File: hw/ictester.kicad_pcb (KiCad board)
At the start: 4 copper layers, 78.2 x 91.4 mm, 71 parts, among them J1 Conn_01x12_Pin, J2 Conn_01x12_Pin, J3 Conn_01x01_Pin, J4 Conn_01x01_Pin, J6 Conn_01x06_Pin, J7 Conn_01x04_Pin, J8 Conn_02x05_Odd_Even, J9 USB_B_Micro, U1 ATmega1284-A, U2 CP2102N-Axx-xQFN28, U3 CDSOT236-0504C, U4 MAX14662, U5 MAX14662, U6 MAX14662, U7 MAX14662, U8 MAX14662, U9 ZIF24, Y1 20MHz

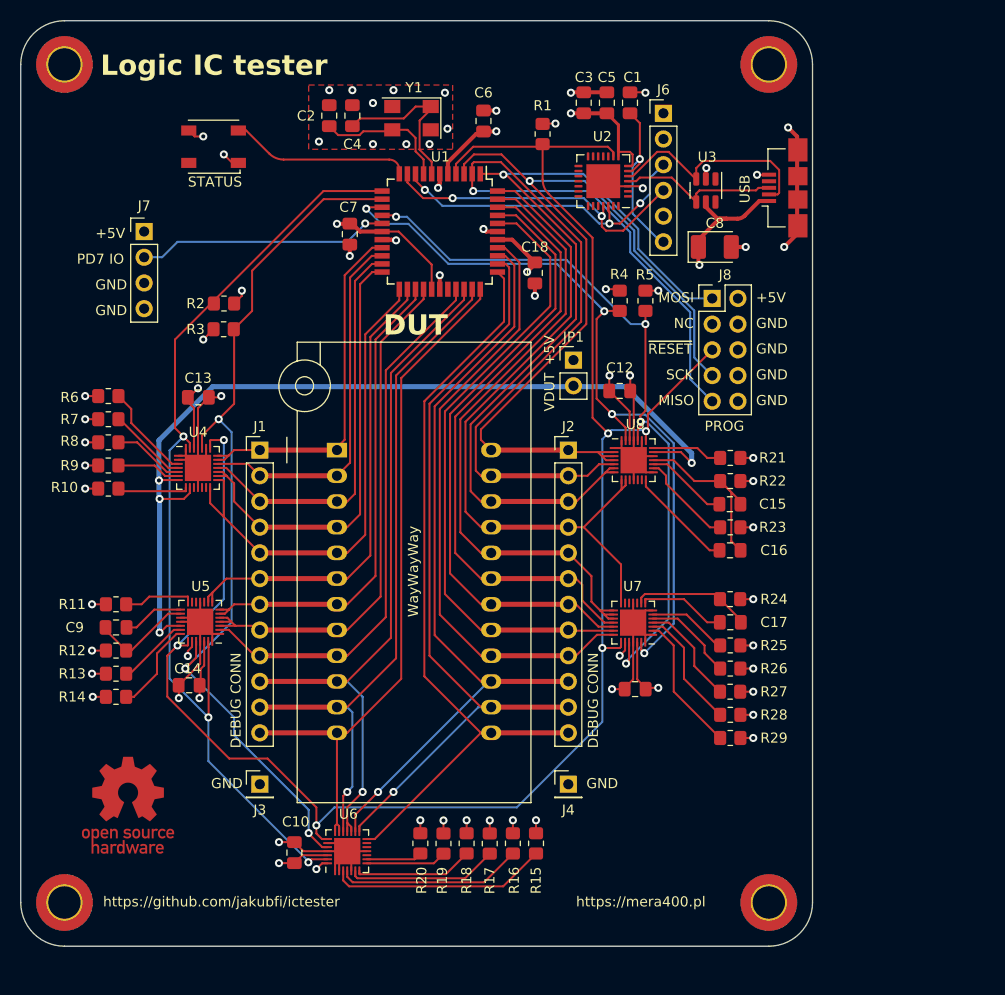
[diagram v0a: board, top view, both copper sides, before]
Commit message: H/W v3
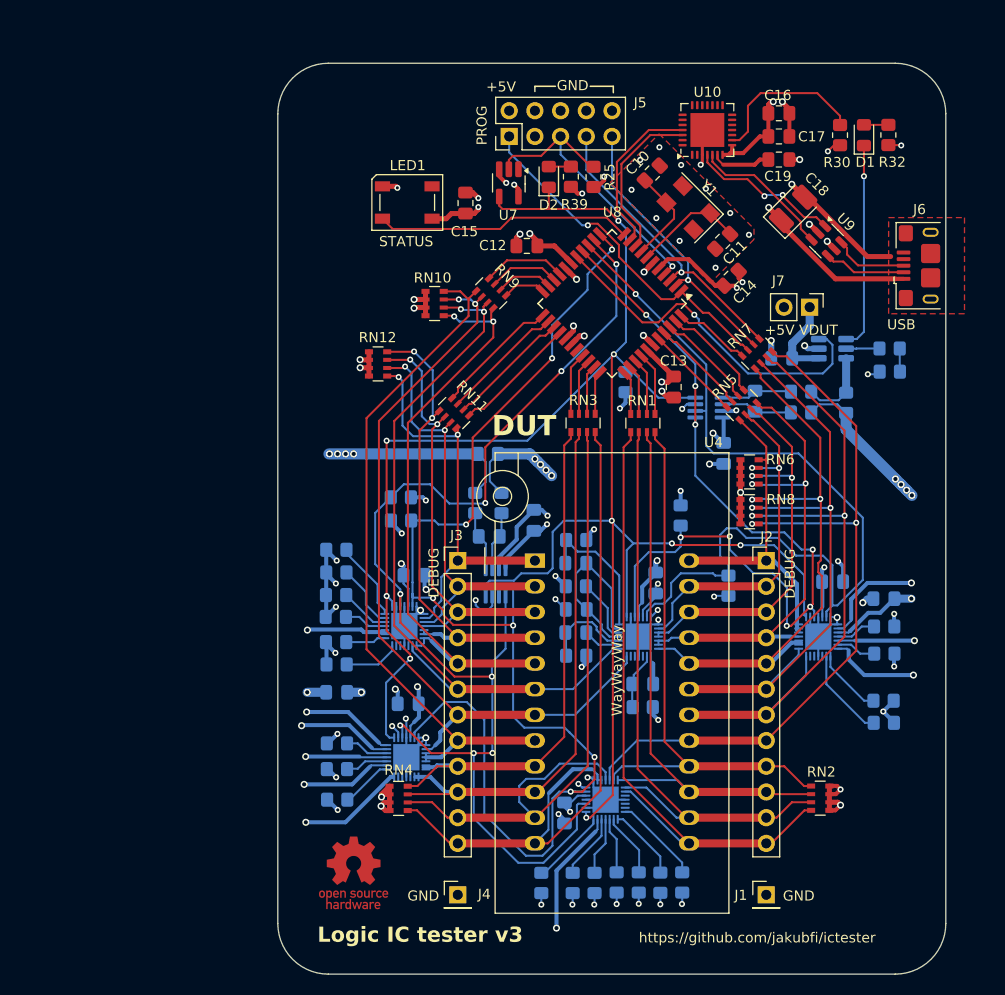
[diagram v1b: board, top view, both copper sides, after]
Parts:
- removed H1, H2, H3, H4: MountingHole_Pad, MountingHole:MountingHole_3.2mm_M3_DIN965_Pad_TopBottom
- removed J8: Conn_02x05_Odd_Even, Connector_PinHeader_2.54mm:PinHeader_2x05_P2.54mm_Vertical
- removed J9: USB_B_Micro, Connector_USB:USB_Micro-B_Amphenol_10104110_Horizontal
- removed JP1: Jumper_2_Open, Connector_PinHeader_2.54mm:PinHeader_1x02_P2.54mm_Vertical
- added C19: 100n, Capacitor_SMD:C_0805_2012Metric_Pad1.18x1.45mm_HandSolder, F.Cu at (176.5, 64.5)
- added C20: 100n, Capacitor_SMD:C_0805_2012Metric_Pad1.18x1.45mm_HandSolder, B.Cu at (176.8, 84.2)
- added C21: 1u, Capacitor_SMD:C_0805_2012Metric_Pad1.18x1.45mm_HandSolder, B.Cu at (186.9, 107.9)
- added C22: 1u, Capacitor_SMD:C_0805_2012Metric_Pad1.18x1.45mm_HandSolder, B.Cu at (132.8, 117.2)
- added C23: 100n, Capacitor_SMD:C_0805_2012Metric_Pad1.18x1.45mm_HandSolder, B.Cu at (174.2, 88.4)
- added C24: 100n, Capacitor_SMD:C_0805_2012Metric_Pad1.18x1.45mm_HandSolder, B.Cu at (147.9, 101.8)
- added C25: 100n, Capacitor_SMD:C_0805_2012Metric_Pad1.18x1.45mm_HandSolder, B.Cu at (171.1, 93.5)
- added C26: 100n, Capacitor_SMD:C_0805_2012Metric_Pad1.18x1.45mm_HandSolder, B.Cu at (152.3, 100.2)
- added D1: RED, LED_SMD:LED_0805_2012Metric_Pad1.15x1.40mm_HandSolder, F.Cu at (184.9, 62.1)
- added D2: ORANGE, LED_SMD:LED_0805_2012Metric_Pad1.15x1.40mm_HandSolder, F.Cu at (153.8, 66.2)
- added J5: Conn_02x05_Odd_Even, Connector_PinHeader_2.54mm:PinHeader_2x05_P2.54mm_Vertical, F.Cu at (149.9, 62.2)
- added R30: 4k7, Resistor_SMD:R_0805_2012Metric_Pad1.20x1.40mm_HandSolder, F.Cu at (182.6, 62.1)
- added R31: 133k, Resistor_SMD:R_0805_2012Metric_Pad1.20x1.40mm_HandSolder, B.Cu at (187.5, 83.2)
- added R32: 1k0, Resistor_SMD:R_0805_2012Metric_Pad1.20x1.40mm_HandSolder, F.Cu at (187.3, 62.1)
- added R33: 200m, Resistor_SMD:R_0805_2012Metric_Pad1.20x1.40mm_HandSolder, B.Cu at (183.2, 88.5)
- added R34: 200m, Resistor_SMD:R_0805_2012Metric_Pad1.20x1.40mm_HandSolder, B.Cu at (147.8, 93.6)
- added R35: 47, Resistor_SMD:R_0805_2012Metric_Pad1.20x1.40mm_HandSolder, B.Cu at (178.7, 87.5)
- added R36: 47, Resistor_SMD:R_0805_2012Metric_Pad1.20x1.40mm_HandSolder, B.Cu at (178.7, 89.5)
- added R37: 47, Resistor_SMD:R_0805_2012Metric_Pad1.20x1.40mm_HandSolder, B.Cu at (146.5, 98.5)
- added R38: 47, Resistor_SMD:R_0805_2012Metric_Pad1.20x1.40mm_HandSolder, B.Cu at (149.1, 98.5)
- added R39: 1k0, Resistor_SMD:R_0805_2012Metric_Pad1.20x1.40mm_HandSolder, F.Cu at (156.0, 66.2)
- added R40: 4k7, Resistor_SMD:R_0805_2012Metric_Pad1.20x1.40mm_HandSolder, B.Cu at (161.3, 86.5)
- added R41: 0, Resistor_SMD:R_0805_2012Metric_Pad1.20x1.40mm_HandSolder, B.Cu at (187.5, 85.5)
- added RN1: 120, Resistor_SMD:R_Array_Convex_4x0603, F.Cu at (163.1, 90.6)
- added RN10: 1M, Resistor_SMD:R_Array_Convex_4x0603, F.Cu at (142.5, 78.7)
- added RN11: 120, Resistor_SMD:R_Array_Convex_4x0603, F.Cu at (144.4, 89.6)
- added RN12: 1M, Resistor_SMD:R_Array_Convex_4x0603, F.Cu at (136.9, 84.7)
- added RN2: 1M, Resistor_SMD:R_Array_Convex_4x0603, F.Cu at (180.6, 127.6)
- added RN3: 120, Resistor_SMD:R_Array_Convex_4x0603, F.Cu at (157.2, 90.5)
- added RN4: 1M, Resistor_SMD:R_Array_Convex_4x0603, F.Cu at (138.9, 127.6)
- added RN5: 120, Resistor_SMD:R_Array_Convex_4x0603, F.Cu at (172.8, 88.8)
- added RN6: 1M, Resistor_SMD:R_Array_Convex_4x0603, F.Cu at (173.6, 95.4)
- added RN7: 120, Resistor_SMD:R_Array_Convex_4x0603, F.Cu at (174.4, 83.7)
- added RN8: 1M, Resistor_SMD:R_Array_Convex_4x0603, F.Cu at (173.6, 99.3)
- added RN9: 120, Resistor_SMD:R_Array_Convex_4x0603, F.Cu at (148.1, 77.7)
- added U10: CP2102N, Package_DFN_QFN:QFN-28-1EP_5x5mm_P0.5mm_EP3.35x3.35mm, F.Cu at (169.4, 61.6)
- added U11: TPS2553, Package_TO_SOT_SMD:SOT-23-6_Handsoldering, B.Cu at (181.8, 83.2)
- added U12: INA236, Package_TO_SOT_SMD:SOT-23-8_Handsoldering, B.Cu at (169.6, 89.0)
- added U13: INA236, Package_TO_SOT_SMD:SOT-23-8_Handsoldering, B.Cu at (148.5, 106.2)
- C1, R10, R11, R12, R13, R14, R15, R16, R17, R18, R19, R2, R20, R21, R22, R23, R24, R26, R27, R28, R29, R3, R4, R5, R6, R7, R8, R9, U5, U6: moved to B.Cu
- C10, C11: value 100n -> 22p
- C15, C17: value 470p -> 100n
- C16: value 470p -> 1u
- C18: value 100n -> 10u; footprint Capacitor_SMD:C_0805_2012Metric_Pad1.18x1.45mm_HandSolder -> Capacitor_Tantalum_SMD:CP_EIA-3528-21_Kemet-B_Pad1.50x2.35mm_HandSolder
- C2, C4: value 22p -> 100n; moved to B.Cu
- C3, C6, C7: value 100n -> 470p; moved to B.Cu
- C5: value 1u -> 100p; moved to B.Cu
- C8: value 10u -> 100n; footprint Capacitor_Tantalum_SMD:CP_EIA-3528-21_Kemet-B_Pad1.50x2.35mm_HandSolder -> Capacitor_SMD:C_0805_2012Metric_Pad1.18x1.45mm_HandSolder; moved to B.Cu
- C9: value 470p -> 100n; moved to B.Cu
- J1: value Conn_01x12_Pin -> Conn_01x01_Pin; footprint Connector_PinHeader_2.54mm:PinHeader_1x12_P2.54mm_Vertical -> Connector_PinHeader_2.54mm:PinHeader_1x01_P2.54mm_Vertical
- J3: value Conn_01x01_Pin -> Conn_01x12_Pin; footprint Connector_PinHeader_2.54mm:PinHeader_1x01_P2.54mm_Vertical -> Connector_PinHeader_2.54mm:PinHeader_1x12_P2.54mm_Vertical
- J6: value Conn_01x06_Pin -> USB_B_Micro; footprint Connector_PinHeader_2.54mm:PinHeader_1x06_P2.54mm_Vertical -> Connector_USB:USB_Micro-B_Amphenol_10118193-0001LF_Horizontal
- J7: value Conn_01x04_Pin -> Conn_02x01; footprint Connector_PinHeader_2.54mm:PinHeader_1x04_P2.54mm_Vertical -> Connector_PinHeader_2.54mm:PinHeader_1x02_P2.54mm_Vertical
- R1: value 10k -> 4k7; moved to B.Cu
- R25: value 4k7 -> 10k
- U1: value ATmega1284-A -> MAX14662; footprint Package_QFP:TQFP-44_10x10mm_P0.8mm -> Package_DFN_QFN:QFN-28-1EP_4x4mm_P0.4mm_EP2.6x2.6mm; moved to B.Cu
- U2: value CP2102N-Axx-xQFN28 -> MAX14662; footprint Package_DFN_QFN:QFN-28-1EP_5x5mm_P0.5mm_EP3.35x3.35mm -> Package_DFN_QFN:QFN-28-1EP_4x4mm_P0.4mm_EP2.6x2.6mm; moved to B.Cu
- U3: value CDSOT236-0504C -> MAX14662; footprint Package_TO_SOT_SMD:SOT-23-6 -> Package_DFN_QFN:QFN-28-1EP_4x4mm_P0.4mm_EP2.6x2.6mm; moved to B.Cu
- U4: value MAX14662 -> ZIF24; footprint Package_DFN_QFN:QFN-28-1EP_4x4mm_P0.4mm_EP2.6x2.6mm -> Socket:DIP_Socket-24_W11.9_W12.7_W15.24_W17.78_W18.5_3M_224-1275-00-0602J
- U7: value MAX14662 -> 74LVC1G07; footprint Package_DFN_QFN:QFN-28-1EP_4x4mm_P0.4mm_EP2.6x2.6mm -> Package_TO_SOT_SMD:SOT-23-5_HandSoldering
- U8: value MAX14662 -> ATmega1284-A; footprint Package_DFN_QFN:QFN-28-1EP_4x4mm_P0.4mm_EP2.6x2.6mm -> Package_QFP:TQFP-44_10x10mm_P0.8mm
- U9: value ZIF24 -> USBLC6-2SC6; footprint Socket:DIP_Socket-24_W11.9_W12.7_W15.24_W17.78_W18.5_3M_224-1275-00-0602J -> Package_TO_SOT_SMD:SOT-23-6
- moved C10 75.9 mm to (164.0, 65.8), turned to 45 degrees
- moved R3 74.8 mm to (186.9, 118.0)
- moved R2 73.9 mm to (186.9, 113.3), turned to 0 degrees
- moved C2 72.7 mm to (155.3, 129.1)
- moved C14 67.0 mm to (171.8, 76.2), turned to -135 degrees
- moved J1 66.6 mm to (175.3, 137.2)
- moved J7 66.2 mm to (179.6, 79.1), turned to -90 degrees
- moved R10 65.3 mm to (162.7, 135.9), turned to -90 degrees
- moved R9 65.0 mm to (160.5, 135.9), turned to -90 degrees
- moved R7 64.8 mm to (156.1, 136.0), turned to -90 degrees
- moved R8 64.8 mm to (158.3, 136.0), turned to -90 degrees
- moved R6 64.4 mm to (153.0, 136.0), turned to -90 degrees
- moved U2 61.1 mm to (159.4, 127.8), turned to -90 degrees
- moved R12 60.5 mm to (167.0, 135.9), turned to -90 degrees
- moved R11 60.4 mm to (164.8, 136.0), turned to -90 degrees
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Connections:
- C1 pad 1: Net-(J6-Pin_6) -> +5V
- C10 pad 1: +5V -> Net-(U8-XTAL1)
- C11 pad 1: +5V -> GND
- C11 pad 2: GND -> Net-(U8-XTAL2)
- C12 pad 1: +5V -> GND
- C12 pad 2: GND -> +5V
- C13 pad 1: +5V -> GND
- C13 pad 2: GND -> +5V
- C14 pad 1: +5V -> GND
- C14 pad 2: GND -> +5V
- C15 pad 1: Net-(U8-B5) -> +5V
- C15 pad 2: Net-(U8-B4) -> GND
- C16 pad 1: Net-(U8-B8) -> +5V
- C16 pad 2: Net-(U8-B4) -> GND
- C17 pad 1: Net-(U7-A7) -> +5V
- C17 pad 2: Net-(U7-A8) -> GND
- C18 pad 1: GND -> +5V
- C18 pad 2: +5V -> GND
- C2 pad 1: GND -> +5V
- C2 pad 2: Net-(U1-XTAL1) -> GND
- C3 pad 1: +5V -> Net-(U3-A7)
- C3 pad 2: GND -> Net-(U3-A8)
- C4 pad 1: GND -> +5V
- C4 pad 2: Net-(U1-XTAL2) -> GND
- C5 pad 1: +5V -> GND
- C5 pad 2: GND -> Net-(U3-B2)
- C6 pad 1: GND -> Net-(U3-B1)
- C6 pad 2: +5V -> Net-(U3-B2)
- C7 pad 1: GND -> Net-(U3-B5)
- C7 pad 2: +5V -> Net-(U3-B6)
- C9 pad 1: Net-(U5-B6) -> +5V
- C9 pad 2: Net-(U5-B7) -> GND
- J1 pad 1: ZIF1 -> GND
- J3 pad 1: GND -> ZIF1
- J6 pad 2: GND -> Net-(J6-D-)
- J6 pad 3: TXD -> Net-(J6-D+)
- J6 pad 4: RXD -> unconnected-(J6-ID-Pad4)
- J6 pad 5: unconnected-(J6-Pin_5-Pad5) -> GND
- J6 pad 6: Net-(J6-Pin_6) -> GND
- J7 pad 1: +5V -> Net-(J7-Pin_1)
- J7 pad 2: Net-(J7-Pin_2) -> +5V
- R1 pad 1: +5V -> Net-(U1-A3)
- R1 pad 2: ~{RESET} -> +5V
- R10 pad 1: Net-(U4-A7) -> Net-(U2-B6)
- R11 pad 1: Net-(U5-B8) -> Net-(U2-B7)
- R12 pad 1: Net-(U5-B6) -> Net-(U2-B8)
- R13 pad 1: Net-(U5-B2) -> +5V
- R13 pad 2: +5V -> Net-(U3-B1)
- R14 pad 1: Net-(U5-B1) -> +5V
- R14 pad 2: +5V -> Net-(U3-B3)
- R15 pad 1: Net-(U6-A2) -> +5V
- R15 pad 2: +5V -> Net-(U3-B5)
- R16 pad 1: Net-(U6-A3) -> Net-(U5-B3)
- R17 pad 1: Net-(U6-A5) -> Net-(U5-B5)
- R18 pad 1: Net-(U6-A6) -> Net-(U5-B7)
- R19 pad 1: Net-(U6-A7) -> Net-(U6-B1)
- R2 pad 1: +5V -> Net-(U1-A5)
- R2 pad 2: SDA1 -> +5V
- R20 pad 1: Net-(U6-A8) -> Net-(U6-B2)
- R21 pad 1: Net-(U8-B1) -> Net-(U6-B3)
- R22 pad 1: Net-(U8-B4) -> Net-(U6-B4)
- R23 pad 1: Net-(U8-B6) -> Net-(U6-B7)
- R24 pad 1: Net-(U7-A8) -> Net-(U6-B8)
- R25 pad 1: Net-(U7-A5) -> +5V
- R25 pad 2: +5V -> Net-(J5-Pin_5)
- R26 pad 1: Net-(U7-A4) -> +5V
- R26 pad 2: +5V -> SDA1
- R27 pad 1: Net-(U7-A3) -> +5V
- R27 pad 2: +5V -> SCL1
- R28 pad 1: Net-(U7-A2) -> +5V
- R28 pad 2: +5V -> SDA2
- R29 pad 1: Net-(U7-A1) -> +5V
- R29 pad 2: +5V -> SCL2
- R3 pad 1: +5V -> Net-(U1-A7)
- R3 pad 2: SCL1 -> +5V
- R4 pad 1: +5V -> Net-(U1-A8)
- R4 pad 2: SDA2 -> +5V
- R5 pad 1: +5V -> Net-(U3-A8)
- R5 pad 2: SCL2 -> +5V
- R6 pad 1: Net-(U4-A2) -> Net-(U2-B1)
- R7 pad 1: Net-(U4-A3) -> Net-(U2-B3)
- R8 pad 1: Net-(U4-A4) -> Net-(U2-B4)
- R9 pad 1: Net-(U4-A5) -> Net-(U2-B5)
- U1 pad 1: ZIF22 -> GND
- U1 pad 10: RXD -> unconnected-(U1-NC-Pad10)
- U1 pad 11: Net-(LED1-DIN) -> GND
- U1 pad 12: SDA1 -> unconnected-(U1-NC-Pad12)
- U1 pad 13: SCL1 -> unconnected-(U1-NC-Pad13)
- U1 pad 14: SDA2 -> ZIF18
- U1 pad 15: SCL2 -> ZIF19
- U1 pad 16: Net-(J7-Pin_2) -> ZIF20
- U1 pad 17: +5V -> ZIF20
- U1 pad 18: GND -> ZIF21
- U1 pad 19: ZIF1 -> ZIF24
- U1 pad 2: ZIF23 -> GNDUT
- U1 pad 20: ZIF2 -> ZIF24
- U1 pad 21: ZIF3 -> ZIF24
- U1 pad 22: ZIF4 -> ~{SD}
- U1 pad 23: ZIF5 -> GND
- U1 pad 24: ZIF6 -> SCL2
- U1 pad 25: ZIF7 -> GND
- U1 pad 26: ZIF8 -> +5V
- U1 pad 27: +5V -> SDA2
- U1 pad 29: unconnected-(U1-AREF-Pad29) -> GND
- U1 pad 3: ZIF24 -> VDUT
- U1 pad 4: ~{RESET} -> Net-(U1-A3)
- U1 pad 5: +5V -> GNDUT
- U1 pad 6: GND -> Net-(U1-A5)
- U1 pad 7: Net-(U1-XTAL2) -> GNDUT
- U1 pad 8: Net-(U1-XTAL1) -> Net-(U1-A7)
- U1 pad 9: TXD -> Net-(U1-A8)
- U2 pad 1: unconnected-(U2-~{DCD}-Pad1) -> GND
- U2 pad 11: unconnected-(U2-~{SUSPEND}-Pad11) -> GND
- U2 pad 14: unconnected-(U2-CHR1-Pad14) -> Net-(U2-B8)
- U2 pad 15: unconnected-(U2-CHR0-Pad15) -> Net-(U2-B7)
- U2 pad 16: unconnected-(U2-~{WAKEUP}/GPIO.3-Pad16) -> Net-(U2-B6)
- U2 pad 17: unconnected-(U2-RS485/GPIO.2-Pad17) -> Net-(U2-B5)
- U2 pad 18: unconnected-(U2-~{RXT}/GPIO.1-Pad18) -> Net-(U2-B4)
- U2 pad 19: unconnected-(U2-~{TXT}/GPIO.0-Pad19) -> Net-(U2-B3)
- U2 pad 2: unconnected-(U2-~{RI}/CLK-Pad2) -> ZIF12
- U2 pad 20: unconnected-(U2-GPIO.6-Pad20) -> GNDUT
- U2 pad 21: unconnected-(U2-GPIO.5-Pad21) -> Net-(U2-B1)
- U2 pad 22: unconnected-(U2-GPIO.4-Pad22) -> ~{SD}
- U2 pad 23: unconnected-(U2-~{CTS}-Pad23) -> GND
- U2 pad 24: unconnected-(U2-~{RTS}-Pad24) -> SCL1
- U2 pad 25: RXD -> GND
- U2 pad 26: TXD -> +5V
- U2 pad 27: unconnected-(U2-~{DSR}-Pad27) -> SDA1
- U2 pad 28: unconnected-(U2-~{DTR}-Pad28) -> +5V
- U2 pad 3: GND -> ZIF12
- U2 pad 4: Net-(J9-D+) -> ZIF11
- U2 pad 5: Net-(J9-D-) -> ZIF17
- U2 pad 6: Net-(J6-Pin_6) -> ZIF16
- U2 pad 7: +5V -> ZIF15
- U2 pad 8: +5V -> ZIF14
- U2 pad 9: ~{RESET} -> ZIF13
- U3 pad 1: unconnected-(U3-IO1-Pad1) -> GND
- U3 pad 2: GND -> ZIF23
- U3 pad 3: Net-(J9-D-) -> ZIF22
- U3 pad 4: Net-(J9-D+) -> ZIF22
- U3 pad 5: +5V -> ZIF21
- U3 pad 6: unconnected-(U3-IO4-Pad6) -> ZIF21
- U4 pad 1: GND -> ZIF1
- U4 pad 10: unconnected-(U4-NC-Pad10) -> ZIF10
- U4 pad 11: GND -> ZIF11
- U4 pad 12: unconnected-(U4-NC-Pad12) -> ZIF12
- U4 pad 13: unconnected-(U4-NC-Pad13) -> ZIF13
- U4 pad 14: ZIF5 -> ZIF14
- U4 pad 15: ZIF5 -> ZIF15
- U4 pad 16: ZIF4 -> ZIF16
- U4 pad 17: ZIF4 -> ZIF17
- U4 pad 18: ZIF3 -> ZIF18
- U4 pad 19: ZIF2 -> ZIF19
- U4 pad 2: GND -> ZIF2
- U4 pad 20: ZIF1 -> ZIF20
- U4 pad 21: ZIF1 -> ZIF21
- U4 pad 22: ~{RESET} -> ZIF22
- U4 pad 23: GND -> ZIF23
- U4 pad 24: SCL1 -> ZIF24
- U4 pad 3: Net-(U4-A2) -> ZIF3
- U4 pad 4: Net-(U4-A3) -> ZIF4
- U4 pad 5: Net-(U4-A4) -> ZIF5
- U4 pad 6: Net-(U4-A5) -> ZIF6
- U4 pad 7: +5VD -> ZIF7
- U4 pad 8: Net-(U4-A7) -> ZIF8
- U4 pad 9: +5VD -> ZIF9
- U5 pad 14: Net-(U5-B8) -> GNDUT
- U5 pad 16: Net-(U5-B6) -> VDUT
- U5 pad 17: GND -> Net-(U5-B5)
- U5 pad 18: GND -> GNDUT
- U5 pad 19: +5VD -> Net-(U5-B3)
- U5 pad 2: ZIF9 -> ZIF7
- U5 pad 20: Net-(U5-B2) -> VDUT
- U5 pad 21: Net-(U5-B1) -> GNDUT
- U5 pad 22: ~{RESET} -> ~{SD}
- U5 pad 6: ZIF7 -> ZIF9
- U5 pad 7: ZIF7 -> ZIF9
- U5 pad 8: ZIF6 -> ZIF10
- U5 pad 9: ZIF6 -> ZIF10
- U6 pad 14: ZIF13 -> Net-(U6-B8)
- U6 pad 15: ZIF14 -> Net-(U6-B7)
- U6 pad 16: ZIF15 -> VDUT
- U6 pad 17: ZIF10 -> VDUT
- U6 pad 18: ZIF10 -> Net-(U6-B4)
- U6 pad 19: ZIF11 -> Net-(U6-B3)
- U6 pad 2: GND -> ZIF1
- U6 pad 20: ZIF12 -> Net-(U6-B2)
- U6 pad 21: ZIF12 -> Net-(U6-B1)
- U6 pad 22: ~{RESET} -> ~{SD}
- U6 pad 28: +5V -> GND
- U6 pad 3: Net-(U6-A2) -> ZIF2
- U6 pad 4: Net-(U6-A3) -> ZIF3
- U6 pad 5: GND -> ZIF4
- U6 pad 6: Net-(U6-A5) -> ZIF4
- U6 pad 7: Net-(U6-A6) -> ZIF5
- U6 pad 8: Net-(U6-A7) -> ZIF5
- U6 pad 9: Net-(U6-A8) -> ZIF6
- U7 pad 1: GND -> unconnected-(U7-NC-Pad1)
- U7 pad 2: Net-(U7-A1) -> Net-(J5-Pin_5)
- U7 pad 3: Net-(U7-A2) -> GND
- U7 pad 4: Net-(U7-A3) -> ~{SD}
- U7 pad 5: Net-(U7-A4) -> +5V
- U8 pad 1: GND -> Net-(J5-Pin_1)
- U8 pad 10: unconnected-(U8-NC-Pad10) -> USB_RXD
- U8 pad 11: GND -> Net-(LED1-DIN)
- U8 pad 12: unconnected-(U8-NC-Pad12) -> SDA1
- U8 pad 13: unconnected-(U8-NC-Pad13) -> SCL1
- U8 pad 14: Net-(U8-B8) -> SDA2
- U8 pad 15: GND -> SCL2
- U8 pad 16: Net-(U8-B6) -> VDUT_EN
- U8 pad 17: Net-(U8-B5) -> +5V
- U8 pad 18: Net-(U8-B4) -> GND
- U8 pad 19: GND -> Net-(RN9-R1.2)
- U8 pad 2: ZIF24 -> Net-(J5-Pin_9)
- U8 pad 20: +5VD -> Net-(RN9-R2.2)
- U8 pad 21: Net-(U8-B1) -> Net-(RN9-R3.2)
- U8 pad 22: ~{RESET} -> Net-(RN9-R4.2)
- U8 pad 23: GND -> Net-(RN11-R1.2)
- U8 pad 24: SCL2 -> Net-(RN11-R2.2)
- U8 pad 25: GND -> Net-(RN11-R3.2)
- U8 pad 26: +5V -> Net-(RN11-R4.2)
- U8 pad 27: SDA2 -> +5V
- U8 pad 29: GND -> unconnected-(U8-AREF-Pad29)
- U8 pad 3: ZIF24 -> Net-(J5-Pin_7)
- U8 pad 4: ZIF24 -> Net-(J5-Pin_5)
- U8 pad 5: ZIF23 -> +5V
- U8 pad 6: ZIF22 -> GND
- U8 pad 7: ZIF22 -> Net-(U8-XTAL2)
- U8 pad 8: ZIF21 -> Net-(U8-XTAL1)
- U8 pad 9: ZIF21 -> USB_TXD
- U9 pad 1: ZIF1 -> Net-(U10-D+)
- U9 pad 2: ZIF2 -> GND
- U9 pad 3: ZIF3 -> Net-(U10-D-)
- U9 pad 4: ZIF4 -> Net-(J6-D-)
- U9 pad 5: ZIF5 -> +5V
- U9 pad 6: ZIF6 -> Net-(J6-D+)
- Y1 pad 1: Net-(U1-XTAL2) -> Net-(U8-XTAL2)
- Y1 pad 3: Net-(U1-XTAL1) -> Net-(U8-XTAL1)
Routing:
- net ~{SD}: track 0.00 -> 198.1 mm, vias 0 -> 9
- net ~{RESET}: track 182.4 -> 0.00 mm, vias 6 -> 0
- net +5VD: track 89.8 -> 0.00 mm, vias 4 -> 0
- net GNDUT: track 0.00 -> 86.3 mm, vias 0 -> 11
- net ZIF23: track 95.3 -> 35.7 mm, vias 1 -> 2
- net ZIF24: track 87.8 -> 32.7 mm, vias 1 -> 0
- net VDUT: track 0.00 -> 51.4 mm, vias 0 -> 9
- net ZIF22: track 84.8 -> 39.5 mm, vias 1 -> 2
- net VDUT_EN: track 0.00 -> 35.7 mm, vias 0 -> 1
- net Net-(J5-Pin_1): track 0.00 -> 34.7 mm, vias 0 -> 1
- net TXD: track 32.0 -> 0.00 mm, vias 3 -> 0
- net RXD: track 31.4 -> 0.00 mm, vias 2 -> 0
- net SCL1: track 89.4 -> 120.1 mm, vias 3 -> 8
- net SDA1: track 95.8 -> 126.3 mm, vias 3 -> 7
- net Net-(J5-Pin_5): track 0.00 -> 29.8 mm, vias 0 -> 1
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- added copper zone on In1.Cu, net GNDUT
- added copper zone on In2.Cu, net VDUT
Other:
- board size 78.2 x 91.4 mm -> 66 x 90 mm
- board text added: "DEBUG"
- board text added: "Logic IC tester v3"
- board text removed: "DEBUG CONN"
- board text removed: "Logic IC tester"
- board text removed: "MISO"
- board text removed: "MOSI"
- board text removed: "NC"
- board text removed: "PD7 IO"
- board text removed: "SCK"
- board text removed: "https://mera400.pl"
- board text removed: "~{RESET}"
